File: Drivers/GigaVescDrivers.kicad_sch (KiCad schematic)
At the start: 21 parts, among them J1 LogicConn, J2 LogicConn2, J3 HVConn, J4 HV1Conn, J5 HV2Conn, J6 HV3Conn, U8 74LVC1G125GV,125

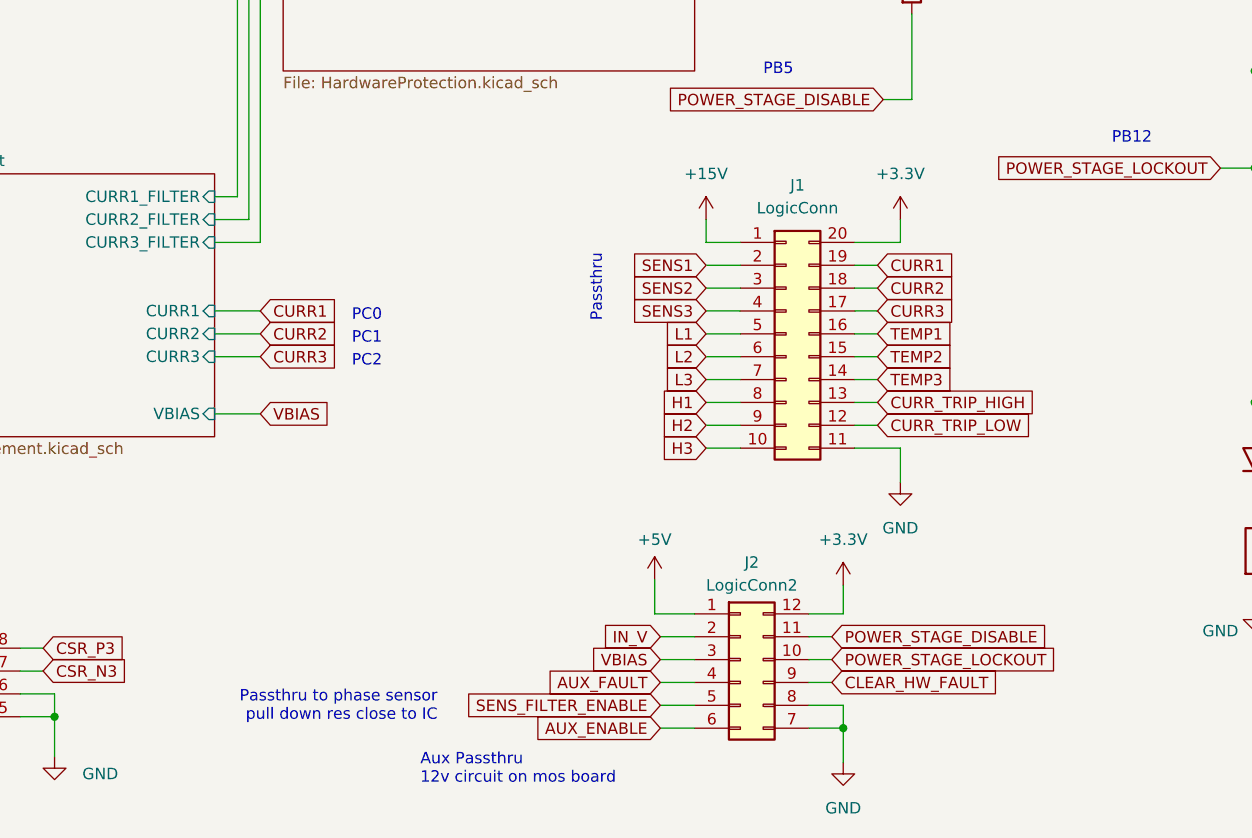
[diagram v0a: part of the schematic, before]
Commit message: driversconnectors
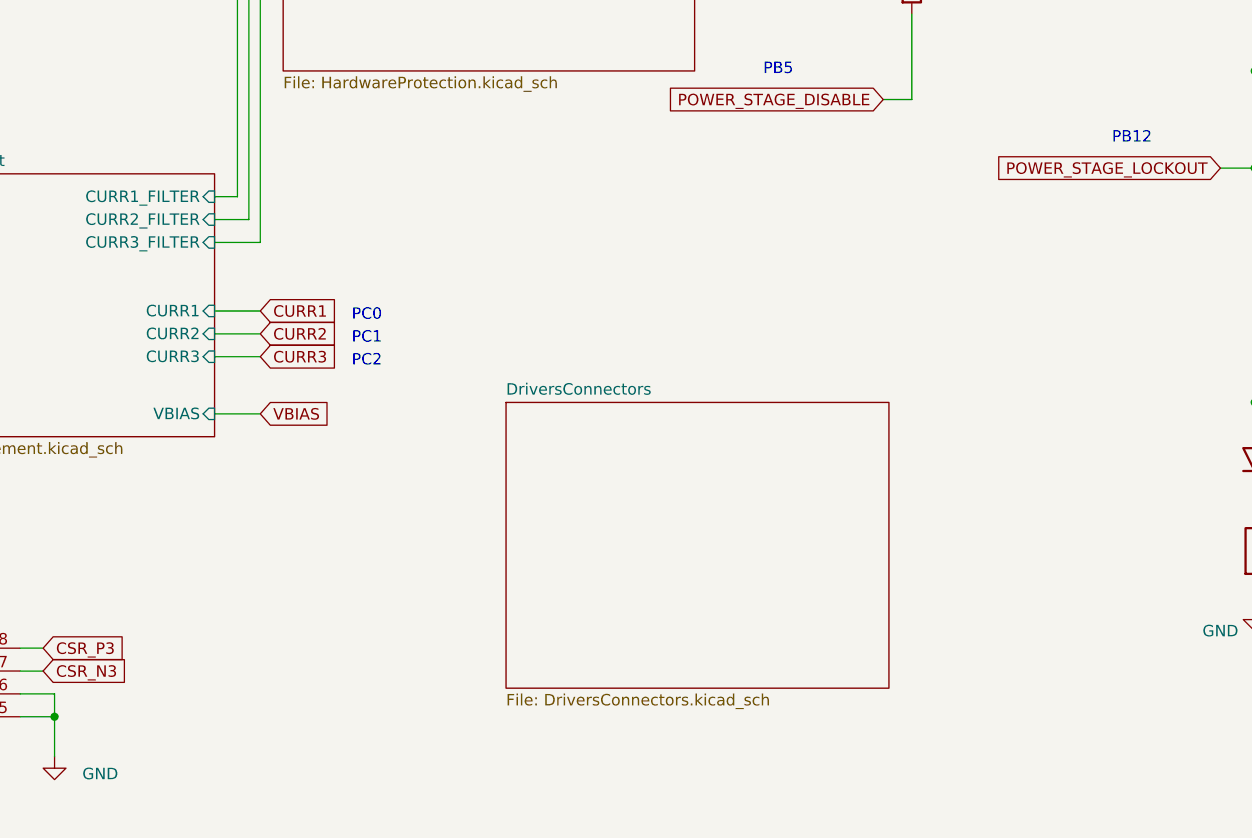
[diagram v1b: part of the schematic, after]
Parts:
- removed J1: LogicConn, Connector_PinSocket_2.54mm:PinSocket_2x10_P2.54mm_Vertical, symbol Connector_Generic:Conn_02x10_Counter_Clockwise
- removed J2: LogicConn2, Connector_PinSocket_2.54mm:PinSocket_2x06_P2.54mm_Vertical, symbol Connector_Generic:Conn_02x06_Counter_Clockwise
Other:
- added sheet DriversConnectors (DriversConnectors.kicad_sch)
- note removed: "Aux Passthru 12v circuit on mos board"
- note removed: "Passthru"
- note removed: "Passthru to phase sensor pull down res close to IC"
